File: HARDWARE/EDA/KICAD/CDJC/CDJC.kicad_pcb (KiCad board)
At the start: 2 copper layers, 63 parts, among them J1 COM_IN, J2 COM_OUT, J3 POWER_IN, J4 POWER_OUT, J5 BIT_OUT, Q1 BC549, SW1 B-SET, U1 74LS04, U2 74LS32, U3 74LS08, U4 74LS08, U5 74LS08, U6 74LS08, U7 74LS32, U8 74LS32, U9 4017

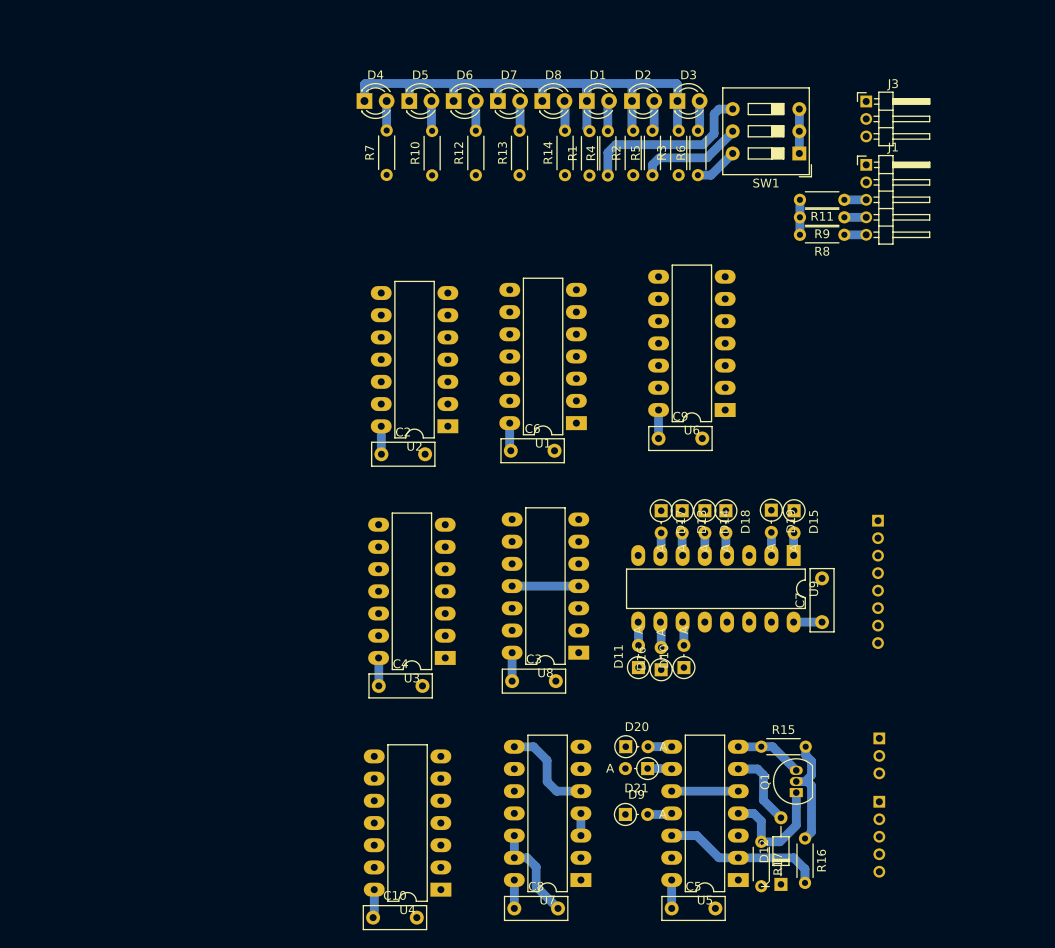
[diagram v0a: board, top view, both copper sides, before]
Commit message: i am crazy
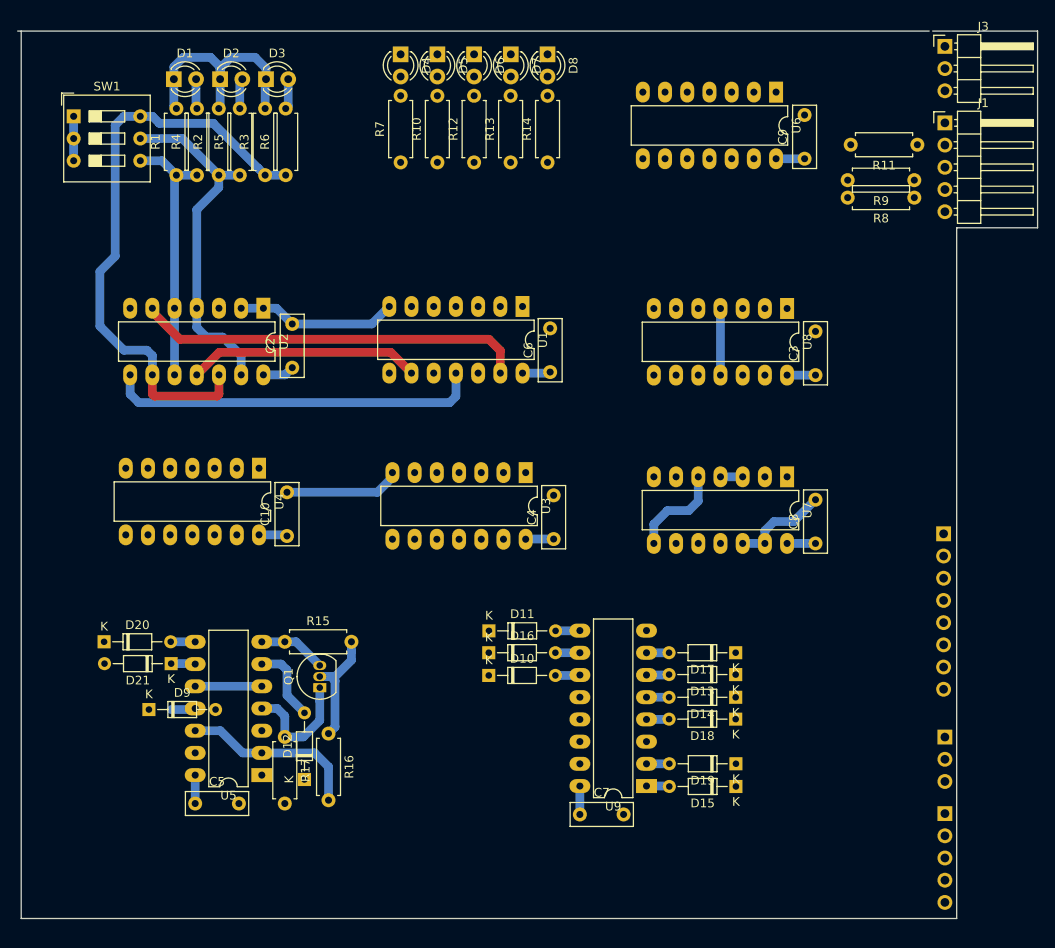
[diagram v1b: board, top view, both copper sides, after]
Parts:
- D10, D11, D13, D14, D15, D16, D17, D18, D19, D20, D21, D9: footprint Diode_THT:D_DO-34_SOD68_P2.54mm_Vertical_AnodeUp -> Diode_THT:D_DO-34_SOD68_P7.62mm_Horizontal
- J1: footprint Connector_PinHeader_2.00mm:PinHeader_1x05_P2.00mm_Horizontal -> Connector_PinHeader_2.54mm:PinHeader_1x05_P2.54mm_Horizontal
- J2: footprint Connector_PinSocket_2.00mm:PinSocket_1x05_P2.00mm_Horizontal -> Connector_PinSocket_2.54mm:PinSocket_1x05_P2.54mm_Horizontal
- J3: footprint Connector_PinHeader_2.00mm:PinHeader_1x03_P2.00mm_Horizontal -> Connector_PinHeader_2.54mm:PinHeader_1x03_P2.54mm_Horizontal
- J4: footprint Connector_PinSocket_2.00mm:PinSocket_1x03_P2.00mm_Horizontal -> Connector_PinSocket_2.54mm:PinSocket_1x03_P2.54mm_Horizontal
- J5: footprint Connector_PinSocket_2.00mm:PinSocket_1x08_P2.00mm_Horizontal -> Connector_PinSocket_2.54mm:PinSocket_1x08_P2.54mm_Horizontal
- R1, R10, R11, R12, R13, R14, R15, R16, R17, R2, R3, R4, R5, R6, R7, R8, R9: footprint Resistor_THT:R_Axial_DIN0204_L3.6mm_D1.6mm_P5.08mm_Horizontal -> Resistor_THT:R_Axial_DIN0207_L6.3mm_D2.5mm_P7.62mm_Horizontal
- moved SW1 83.1 mm to (92.0, 46.8), turned to 0 degrees
- moved D20 60.9 mm to (95.5, 106.8)
- moved D9 55.8 mm to (100.6, 114.6)
- moved U5 55.8 mm to (113.5, 122.1)
- moved C5 55.8 mm to (105.9, 125.3)
- moved D12 55.8 mm to (118.4, 122.6)
- moved D21 55.8 mm to (103.2, 109.3)
- moved Q1 55.8 mm to (120.2, 112.1)
- moved R15 55.8 mm to (116.2, 106.8)
- moved R16 55.8 mm to (121.2, 117.3)
- moved R17 55.8 mm to (116.2, 117.7)
- moved C8 54.1 mm to (176.8, 95.6), turned to 90 degrees
- moved U4 52.5 mm to (113.2, 87.0), turned to 270 degrees
- moved U7 51.8 mm to (173.6, 88.0), turned to 270 degrees
- moved C3 49.3 mm to (176.8, 76.3), turned to 90 degrees
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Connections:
- U2 pad 1: LB_SW -> GNDD
- U2 pad 10: NB_SW -> LB_SW
- U2 pad 11: Net-(U2-Pad11) -> Net-(U1-Pad9)
- U2 pad 12: GNDD -> FB_SW
- U2 pad 13: GNDD -> NB_SW
- U2 pad 2: NB_SW -> GNDD
- U2 pad 3: Net-(U1-Pad9) -> Net-(U2-Pad3)
- U2 pad 4: FB_SW -> NB_SW
- U2 pad 6: Net-(U1-Pad11) -> Net-(U1-Pad13)
- U2 pad 8: Net-(U1-Pad13) -> Net-(U1-Pad11)
- U3 pad 1: Net-(U1-Pad8) -> Net-(U1-Pad12)
- U3 pad 9: Net-(U1-Pad12) -> Net-(U1-Pad8)
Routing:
- net FB_SW: track 5.01 -> 68.2 mm
- net Net-(U1-Pad13): track 0.00 -> 44.6 mm
- net Net-(U1-Pad11): track 0.00 -> 42.8 mm
- net NB_SW: track 12.0 -> 40.2 mm
- net Net-(U1-Pad9): track 0.00 -> 26.6 mm
- net LB_SW: track 20.3 -> 30.1 mm
- net GNDD: track 87.2 -> 79.6 mm
- net Net-(D5-Pad2): track 3.45 -> 0.00 mm
- net Net-(D7-Pad2): track 3.43 -> 0.00 mm
- net Net-(D8-Pad2): track 3.42 -> 0.00 mm
- net Net-(D6-Pad2): track 3.40 -> 0.00 mm
- net Net-(D4-Pad2): track 3.37 -> 0.00 mm
- net MRI: track 2.50 -> 0.00 mm
- net LBLBI: track 2.50 -> 0.00 mm
- net EI: track 2.50 -> 0.00 mm
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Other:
- board outline added: 116.7 x 101.5 mm
